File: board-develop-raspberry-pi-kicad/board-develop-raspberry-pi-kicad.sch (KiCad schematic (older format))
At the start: 32 parts, among them P1 XN1, P2 DOMINO, P3 XN2, P4 CONN_02X20, Q1 2SC1815, U1 MAX485, U2 LTV-817, U3 LM2596, U4 LTV-817

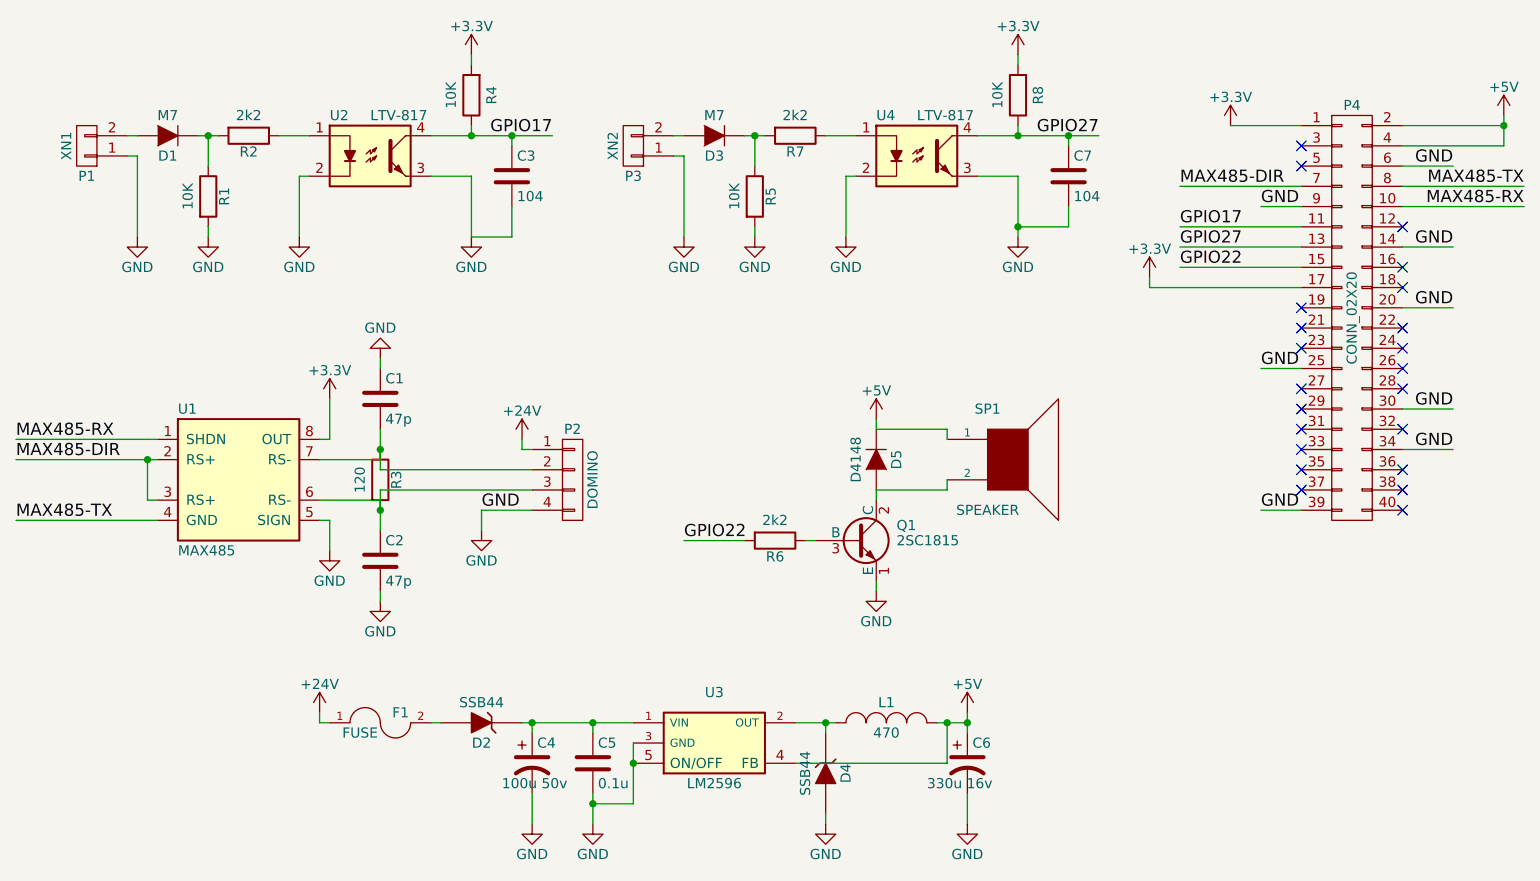
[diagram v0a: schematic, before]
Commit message: backup PCB 1st
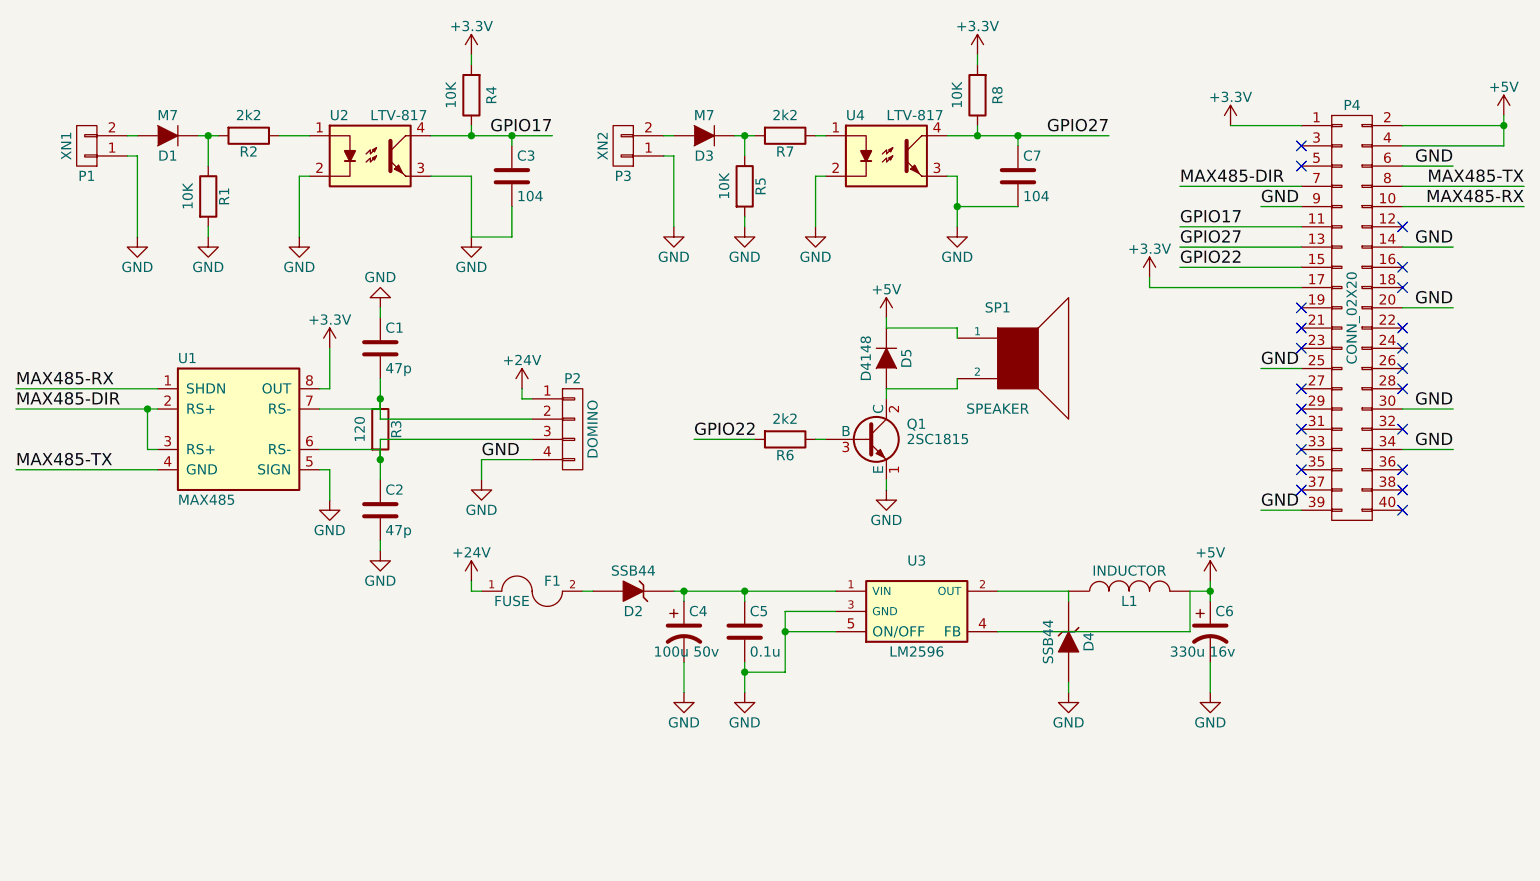
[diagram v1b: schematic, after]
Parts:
- removed L1: 470, Inductors:SELF-WE-PD-XXL, symbol INDUCTOR_SMALL
- added L1: INDUCTOR, Inductors:SELF-WE-PD-XXL, symbol INDUCTOR
- P1, P3: footprint Connect:AK300-2 -> conn:domino-2
- U4: footprint Devices:Optocoupler_SMD_HandSoldering_KPC357_LTV35x_PC357_SingleChannel -> Opto-Devices:Optocoupler_SMD_HandSoldering_KPC357_LTV35x_PC357_SingleChannel
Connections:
- net +5V: now also L1.2
- net at D4.1 (K), U3.2 (OUT): now also L1.1
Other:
- moved on the sheet: C1, C2, C4, C5, C6, D2, D4, D5, P2, Q1, R3, R6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
